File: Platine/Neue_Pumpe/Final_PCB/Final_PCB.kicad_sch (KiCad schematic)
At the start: 20 parts, among them J1 Conn_01x12, J3 Conn_01x10, J4 Conn_01x10, J5 Conn_01x10, J6 Conn_01x08, J7 Conn_01x06, J8 Conn_01x08, J9 Conn_01x06

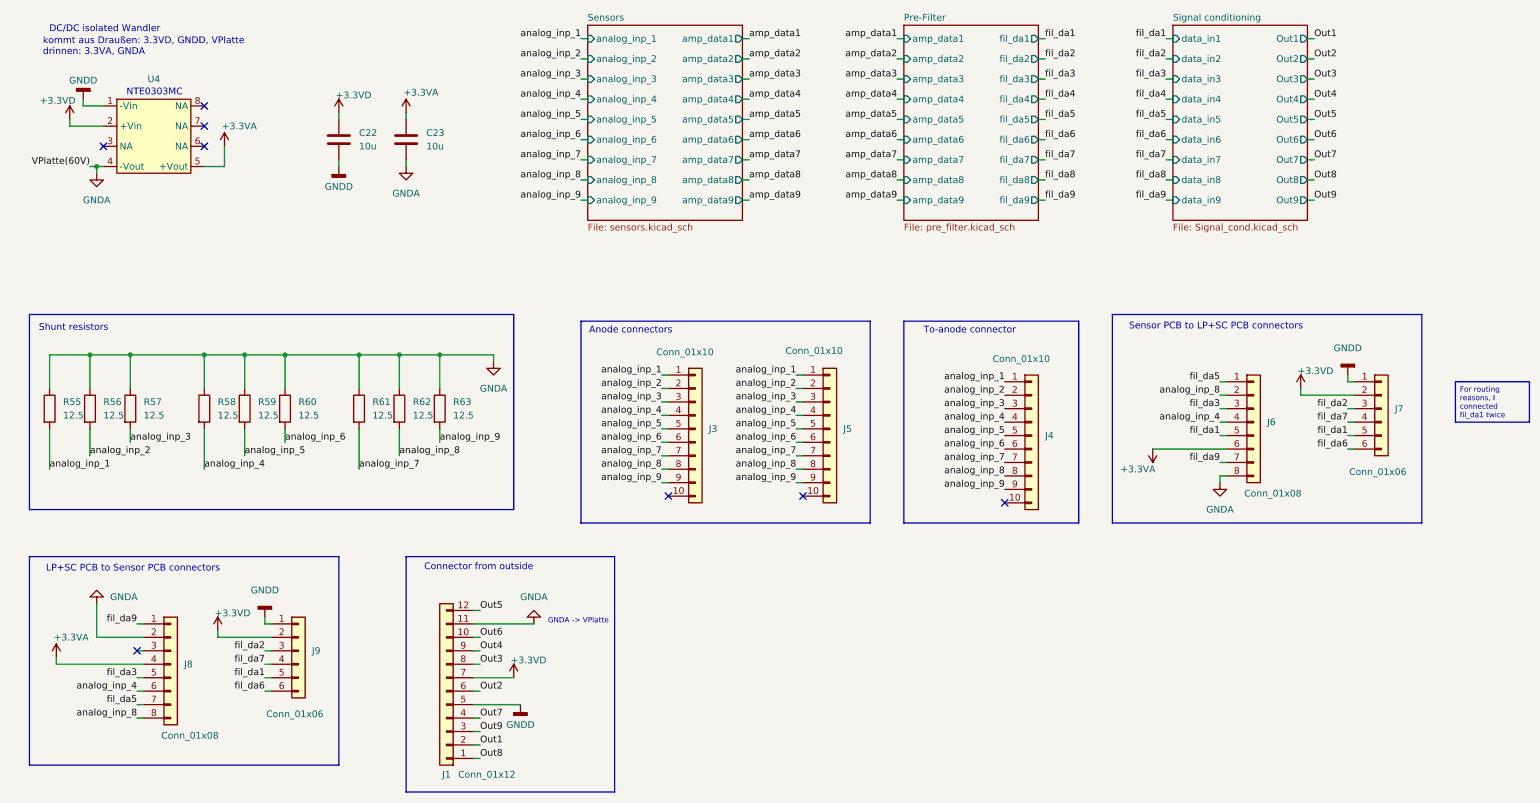
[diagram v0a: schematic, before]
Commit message: final PCB finished
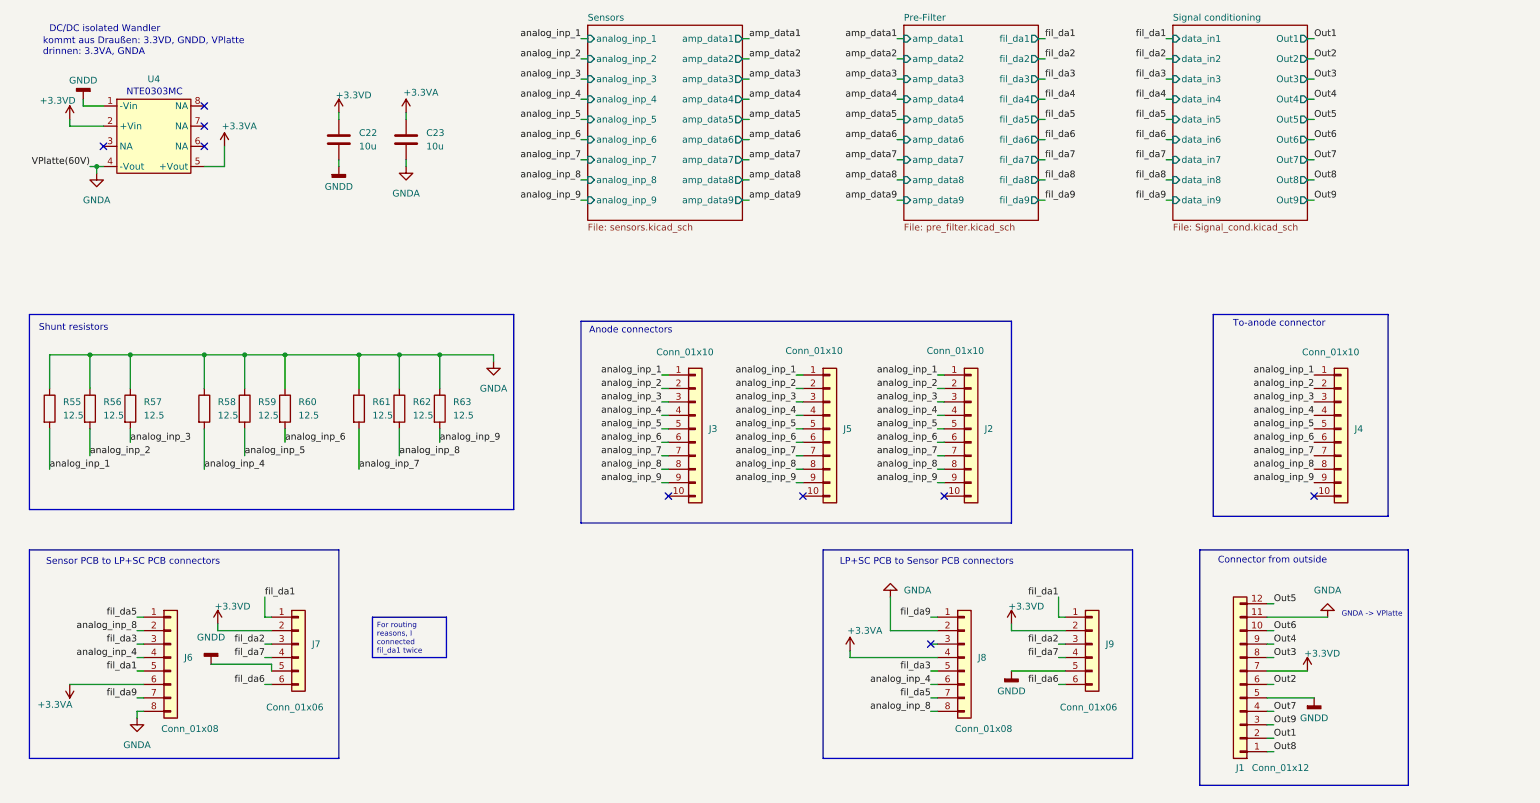
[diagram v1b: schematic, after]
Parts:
- added J2: Conn_01x10, FLE-105-01-G-DV-K-TR:FLE-105-01-X-DV-Y-TR, symbol Connector_Generic:Conn_01x10
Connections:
- net GNDD: now also J7.5 (Pin_5), J9.5 (Pin_5); no longer J7.1 (Pin_1), J9.1 (Pin_1)
- net analog_inp_1: now also J2.1 (Pin_1)
- net analog_inp_2: now also J2.2 (Pin_2)
- net analog_inp_3: now also J2.3 (Pin_3)
- net analog_inp_4: now also J2.4 (Pin_4)
- net analog_inp_5: now also J2.5 (Pin_5)
- net analog_inp_6: now also J2.6 (Pin_6)
- net analog_inp_7: now also J2.7 (Pin_7)
- net analog_inp_8: now also J2.8 (Pin_8)
- net analog_inp_9: now also J2.9 (Pin_9)
- net fil_da1: now also J7.1 (Pin_1), J9.1 (Pin_1); no longer J7.5 (Pin_5), J9.5 (Pin_5)
- no-connect marks 8 -> 9
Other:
- moved on the sheet: J1, J4, J6, J7, J8, J9
